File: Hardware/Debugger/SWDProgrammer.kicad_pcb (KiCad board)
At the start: 4 copper layers, 24.3 x 31 mm, 40 parts, among them J1 USB_C_Receptacle_USB2.0, J2 USB_C_Receptacle_USB2.0, U1 AP2112K-3.3, U2 STM32F103C8Tx, Y1 32.768KHZ, Y2 8Mhz

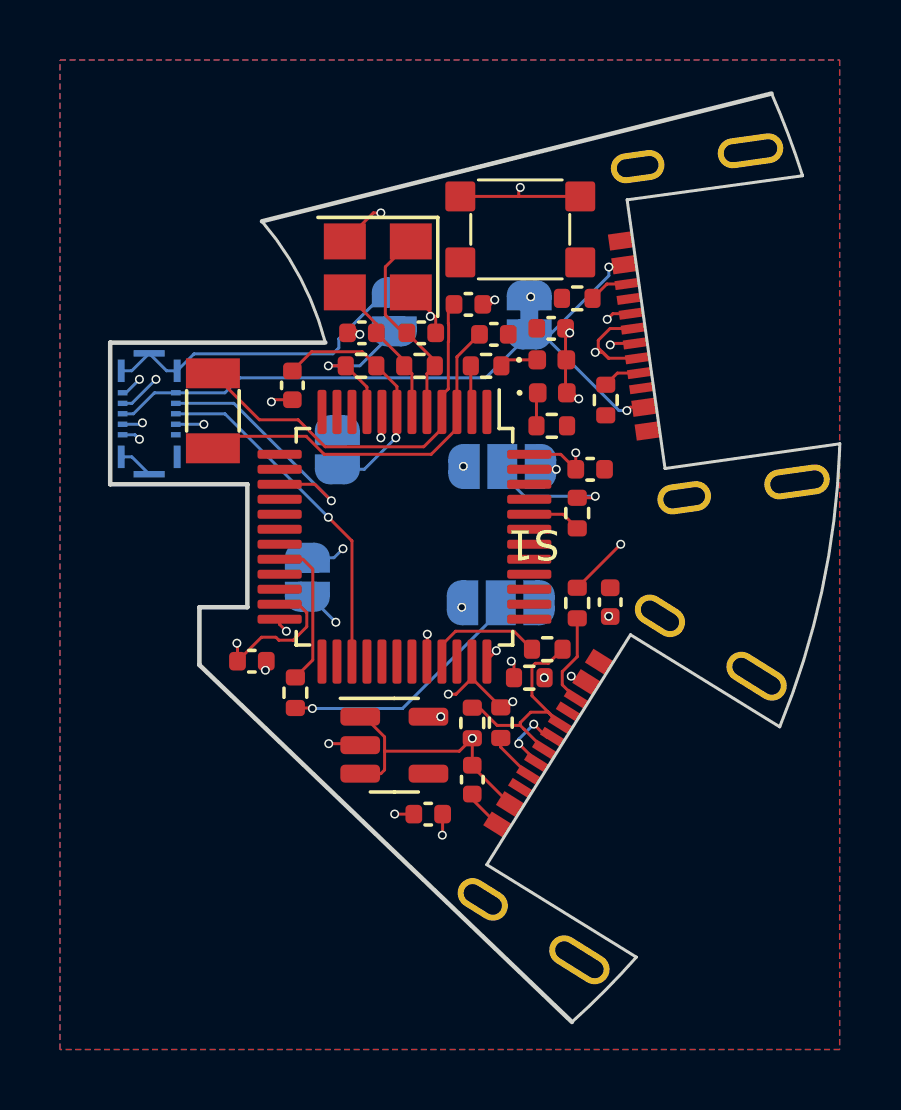
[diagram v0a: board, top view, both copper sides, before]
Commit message: finished debugger and wireless
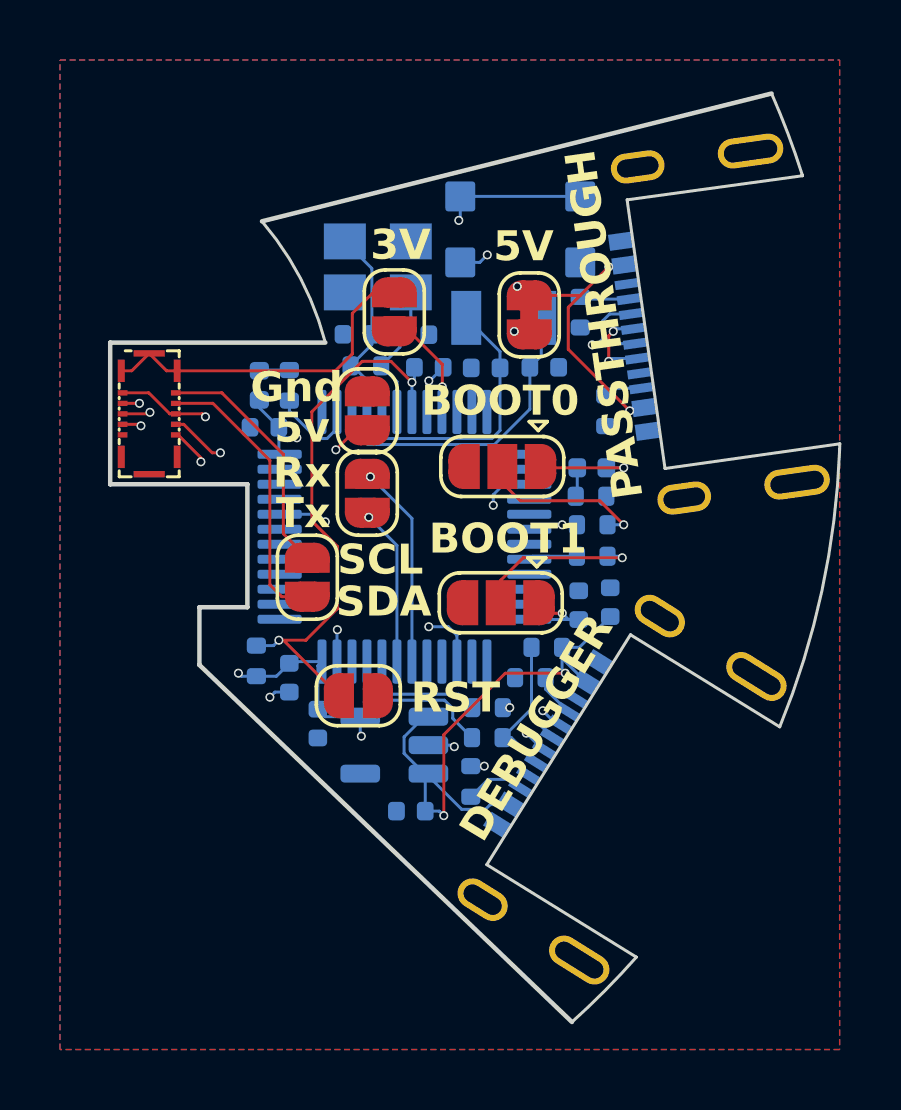
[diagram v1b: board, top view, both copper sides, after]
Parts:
- added JP7: SolderJumper_2_Open, Jumper:SolderJumper-2_P1.3mm_Open_RoundedPad1.0x1.5mm, F.Cu at (141.2, 62.5)
- added JP7: SolderJumper_2_Open, Jumper:SolderJumper-2_P1.3mm_Open_RoundedPad1.0x1.5mm, F.Cu at (141.2, 59.7)
- C1, C10, C11, C2, C3, C4, C5, C6, C7, C8, C9, D1, D2, J1, J2, R1, R10, R11, R12, R13, R2, R3, R4, R5, R6, R7, R8, R9, S1, U1, U2, Y1, Y2: moved to B.Cu
- JP1, JP2, JP3, JP4, JP5, U3: moved to F.Cu
- JP7: renamed from JP1; moved to F.Cu
- moved C8 12.2 mm to (138.7, 68.6), turned to 90 degrees
- moved C9 11.1 mm to (148.3, 66.2), turned to -90 degrees
- moved R2 10.9 mm to (148.8, 64.5), turned to 180 degrees
- moved R4 10.4 mm to (137.6, 68.0), turned to 90 degrees
- moved Y1 10.2 mm to (145.8, 56.6), turned to 0 degrees
- moved C7 10.1 mm to (137.8, 60.2)
- moved D1 9.79 mm to (137.7, 58.9), turned to -90 degrees
- moved JP1 8.23 mm to (140.9, 69.2), turned to 0 degrees
- moved R9 6.93 mm to (144.7, 72.1)
- moved R3 6.59 mm to (138.7, 58.9), turned to -90 degrees
- moved C6 4.76 mm to (139.6, 70.1), turned to 90 degrees
- moved C5 4.59 mm to (143.3, 58.2), turned to 180 degrees
- moved R12 3.87 mm to (149.2, 59.7), turned to 90 degrees
- moved R6 3.56 mm to (145.2, 70.6)
- moved R11 3.54 mm to (147.2, 67.6), turned to 180 degrees
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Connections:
- U2 pad 30: unconnected-(U2-PA9-Pad30) -> /A9
- U2 pad 31: unconnected-(U2-PA10-Pad31) -> /A10
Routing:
- net GND: track 21.6 -> 5.85 mm, vias 13 -> 6
- net 5V: track 28.8 -> 42.4 mm
- net Net-(JP1-A): track 8.35 -> 18.7 mm, vias 1 -> 2
- net Net-(U2-BOOT0): track 1.79 -> 10.8 mm, vias 0 -> 2
- net swc: track 8.49 -> 16.6 mm, vias 1 -> 2
- net 3.3V: track 12.7 -> 19.7 mm, vias 11 -> 6
- net /A9: track 0.00 -> 6.74 mm, vias 0 -> 1
- net /A10: track 0.00 -> 5.20 mm, vias 0 -> 1
- net SDA: track 14.1 -> 9.49 mm, vias 2 -> 0
- net swd: track 11.7 -> 16.2 mm, vias 1 -> 2
- net SCL: track 12.6 -> 8.22 mm, vias 2 -> 0
- net Net-(U2-PC15): track 13.2 -> 9.46 mm
- net Net-(U2-PB2): track 5.09 -> 1.63 mm
- net /BOOT1: track 8.46 -> 5.62 mm
- net /BOOT0: track 4.28 -> 6.30 mm
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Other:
- board text added: "5v"
- board text added: "DEBUGGER"
- board text added: "Gnd"
- board text added: "PASSTHROUGH"
- board text added: "Rx"
- board text added: "Tx"
- board text removed: "PASS TO"
